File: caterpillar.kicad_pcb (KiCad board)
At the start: 2 copper layers, 20.2 x 20.2 mm, 32 parts, among them J1 Conn_ARM_JTAG_SWD_10, M1 Conn_01x02_Pin, M2 *, M3 Conn_01x02_Pin, U1 STBB1-APUR, U2 ASM330LHHTR, U3 DRV8212P, U4 ADP2503ACPZ-3.3-R7, U6 max5419leta+T

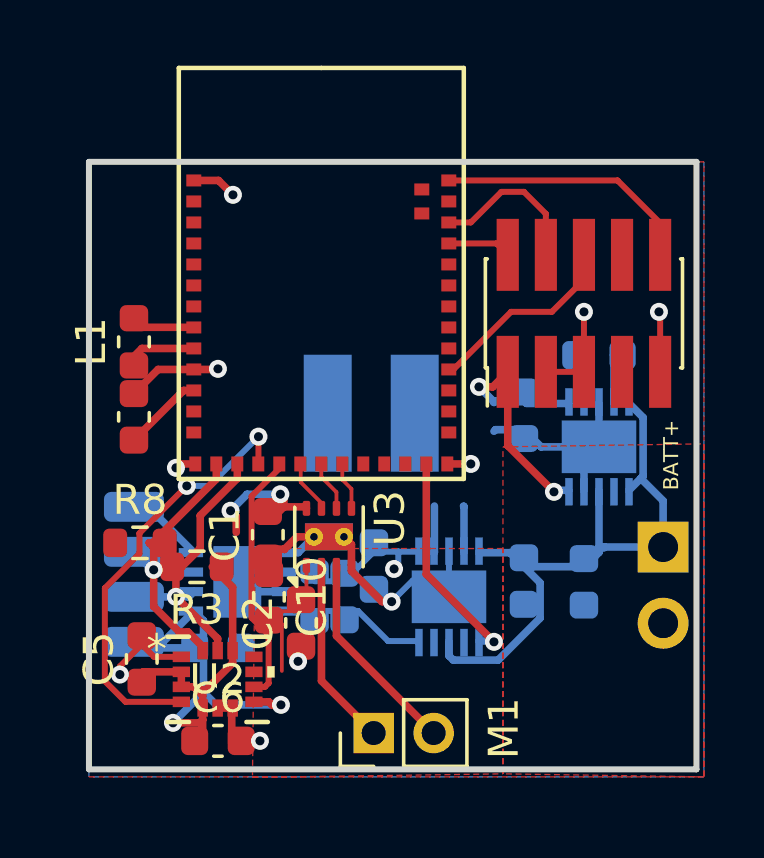
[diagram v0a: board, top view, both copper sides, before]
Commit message: reorganized design a lot for better space organization
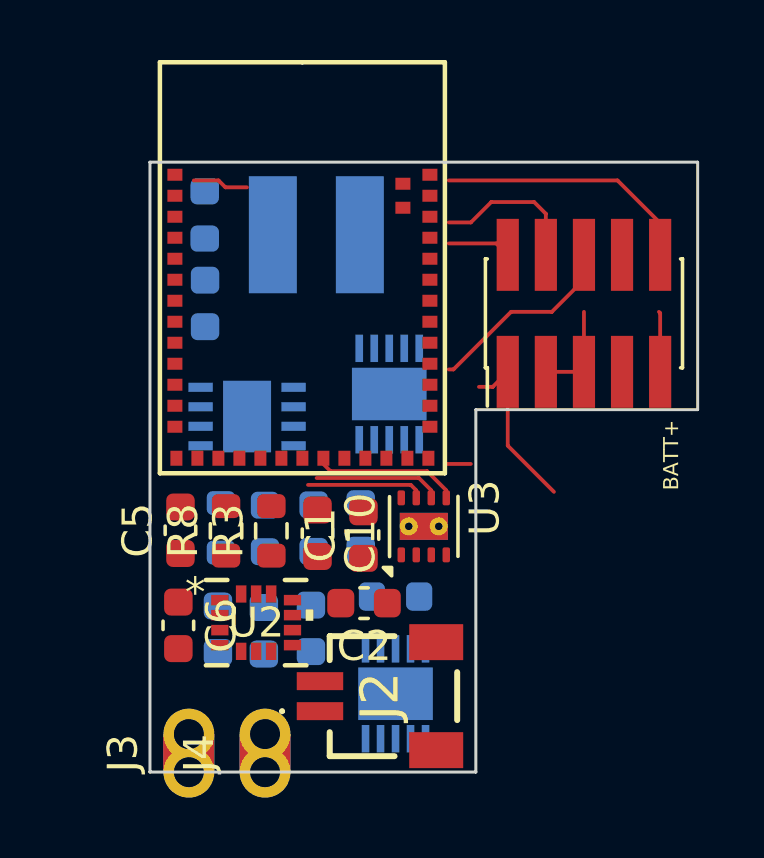
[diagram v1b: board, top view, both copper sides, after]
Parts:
- removed 3.3V1, GND2, SCL1, SDA1: Conn_01x01_Pin, Connector_Wire:SolderWirePad_1x01_SMD_1x2mm
- removed M1: Conn_01x02_Pin, Connector_PinHeader_2.00mm:PinHeader_1x02_P2.00mm_Vertical
- removed M3: Conn_01x02_Pin, Connector_PinHeader_2.54mm:PinHeader_1x02_P2.54mm_Vertical
- added J2: SM02B-SRSS-TB_LF__SN_, SM02B-SRSS-TB:SM02BSRSSTBLFSN, F.Cu at (118.0, 107.8)
- added J3: Castellated_2PTH_P1.27mm, Castellated_2PTH_P1.27mm:Castellated_2PTH_P1.27mm, F.Cu at (111.3, 109.7)
- added J4: Castellated_2PTH_P1.27mm, Castellated_2PTH_P1.27mm:Castellated_2PTH_P1.27mm, F.Cu at (113.9, 109.7)
- C17, L1: moved to B.Cu
- moved U4 10.7 mm to (118.2, 107.7)
- moved L6 10.5 mm to (118.2, 104.5)
- moved C3 9.23 mm to (115.4, 105.5), turned to 90 degrees
- moved C11 8.83 mm to (113.8, 105.6), turned to 90 degrees
- moved U1 7.05 mm to (118.0, 97.7)
- moved C8 6.59 mm to (117.1, 102.2)
- moved L5 6.23 mm to (115.6, 92.4)
- moved U6 5.52 mm to (113.3, 98.5)
- moved L1 4.84 mm to (111.9, 91.8)
- moved C5 4.48 mm to (111.0, 102.3)
- moved C17 4.46 mm to (111.9, 94.7)
- moved C6 4.07 mm to (111.0, 105.5), turned to -90 degrees
- moved R4 3.87 mm to (112.4, 102.2), turned to 90 degrees
- moved C7 3.49 mm to (113.9, 102.2), turned to 90 degrees
- moved C1 3.19 mm to (117.2, 102.4)
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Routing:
- net GND: track 42.9 -> 6.13 mm, vias 10 -> 0
- net +3.3V: track 40.6 -> 5.80 mm, vias 6 -> 0
- net +BATT: track 20.6 -> 0.00 mm
- net /IMU_INT1: track 14.5 -> 0.00 mm, vias 2 -> 0
- net /SDA: track 10.3 -> 0.00 mm, vias 1 -> 0
- net /SCL: track 9.72 -> 0.00 mm, vias 1 -> 0
- net VDC: track 9.37 -> 0.00 mm, vias 1 -> 0
- net /IMU_INT2: track 8.47 -> 0.00 mm
- net /SHDN1: track 7.37 -> 0.00 mm, vias 1 -> 0
- net /OUT2: track 6.93 -> 0.00 mm
- net /OUT1: track 6.31 -> 0.00 mm
- net /FB: track 5.04 -> 0.00 mm
- net /IN2: track 1.61 -> 4.71 mm
- net /IN1: track 1.69 -> 4.24 mm
- net /M_SLP: track 1.77 -> 3.93 mm
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- added copper zone on In1.Cu, net GND
- removed copper zone on F.Cu, net +3.3V
- removed copper zone on F.Cu, net +BATT
- removed copper zone on B.Cu, net GND
- removed copper zone on F.Cu, net VDC
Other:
- board size 20.2 x 20.2 mm -> 18.3 x 20.3 mm
- copper layers 2 -> 4
